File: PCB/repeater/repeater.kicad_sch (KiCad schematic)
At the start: 101 parts, among them J1 TX, J2 RX, J3 Conn_02x03_Counter_Clockwise, SW1 SW_Push, SW2 SW_SPDT, SW3 SW_SPDT, U1 DRA818V, U2 DRA818U, U3 PGA-103, U4 STM32F103C8Tx, U5 LMR33630ADDA, U6 AMS1117-3.3, U7 AMS1117-5.0, Y1 32.768KHz 12.5pF, Y2 8MHz 12pF

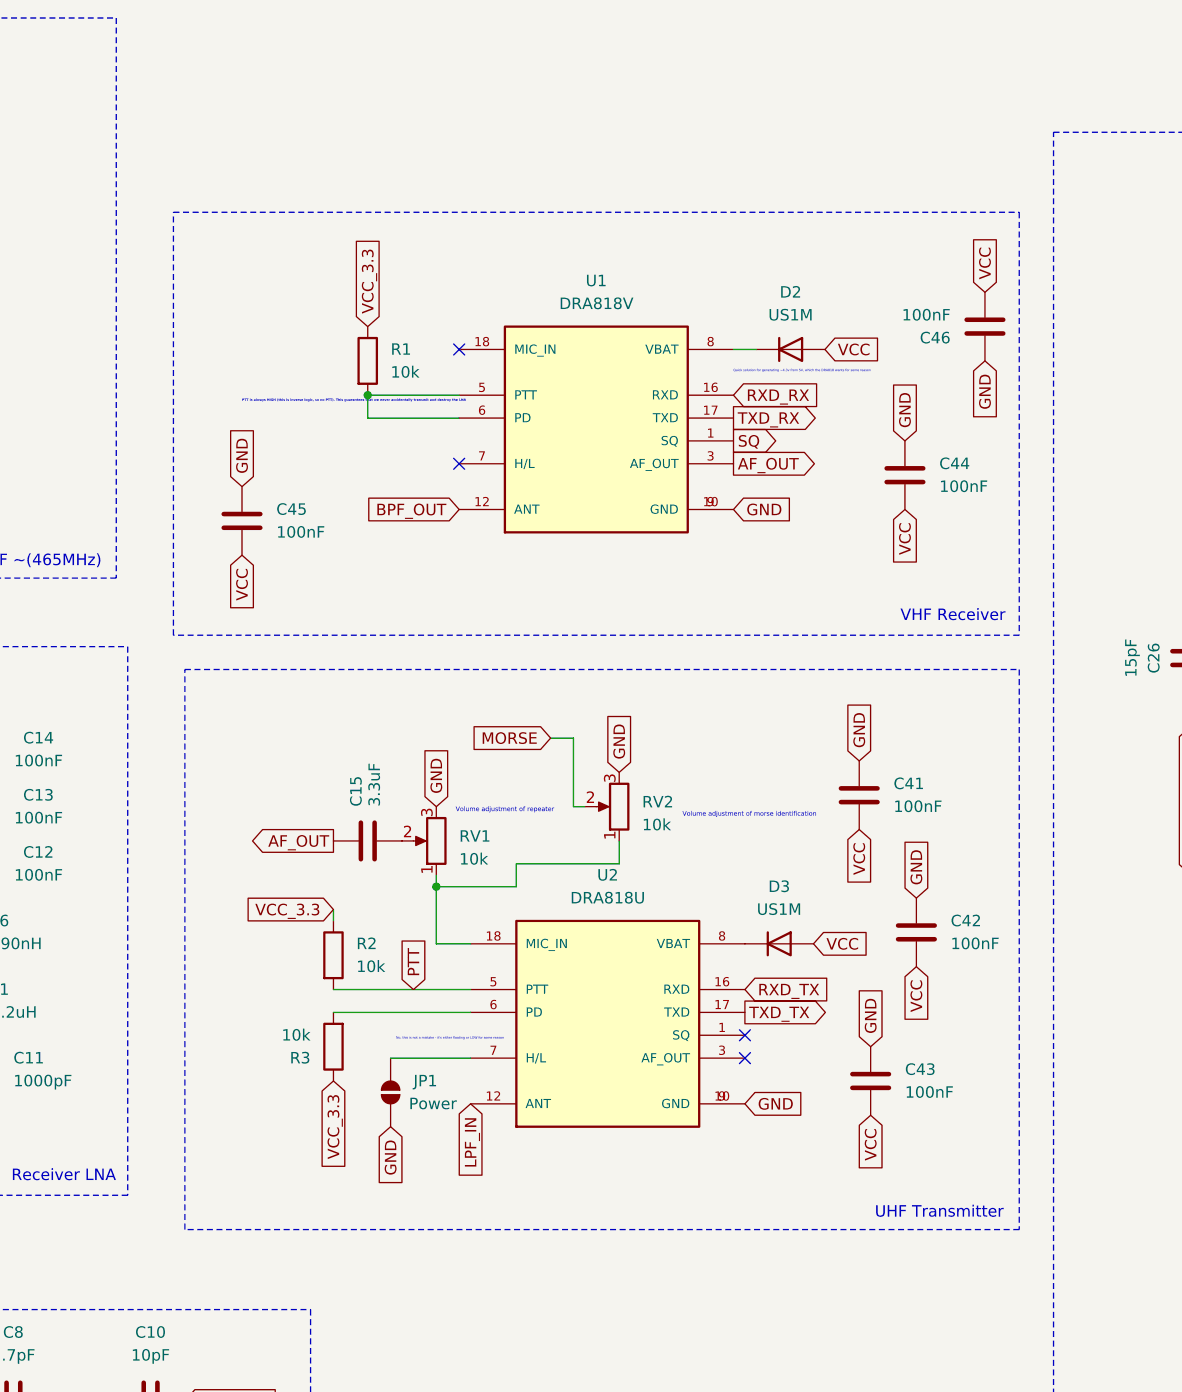
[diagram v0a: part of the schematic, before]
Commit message: Add filter and switch
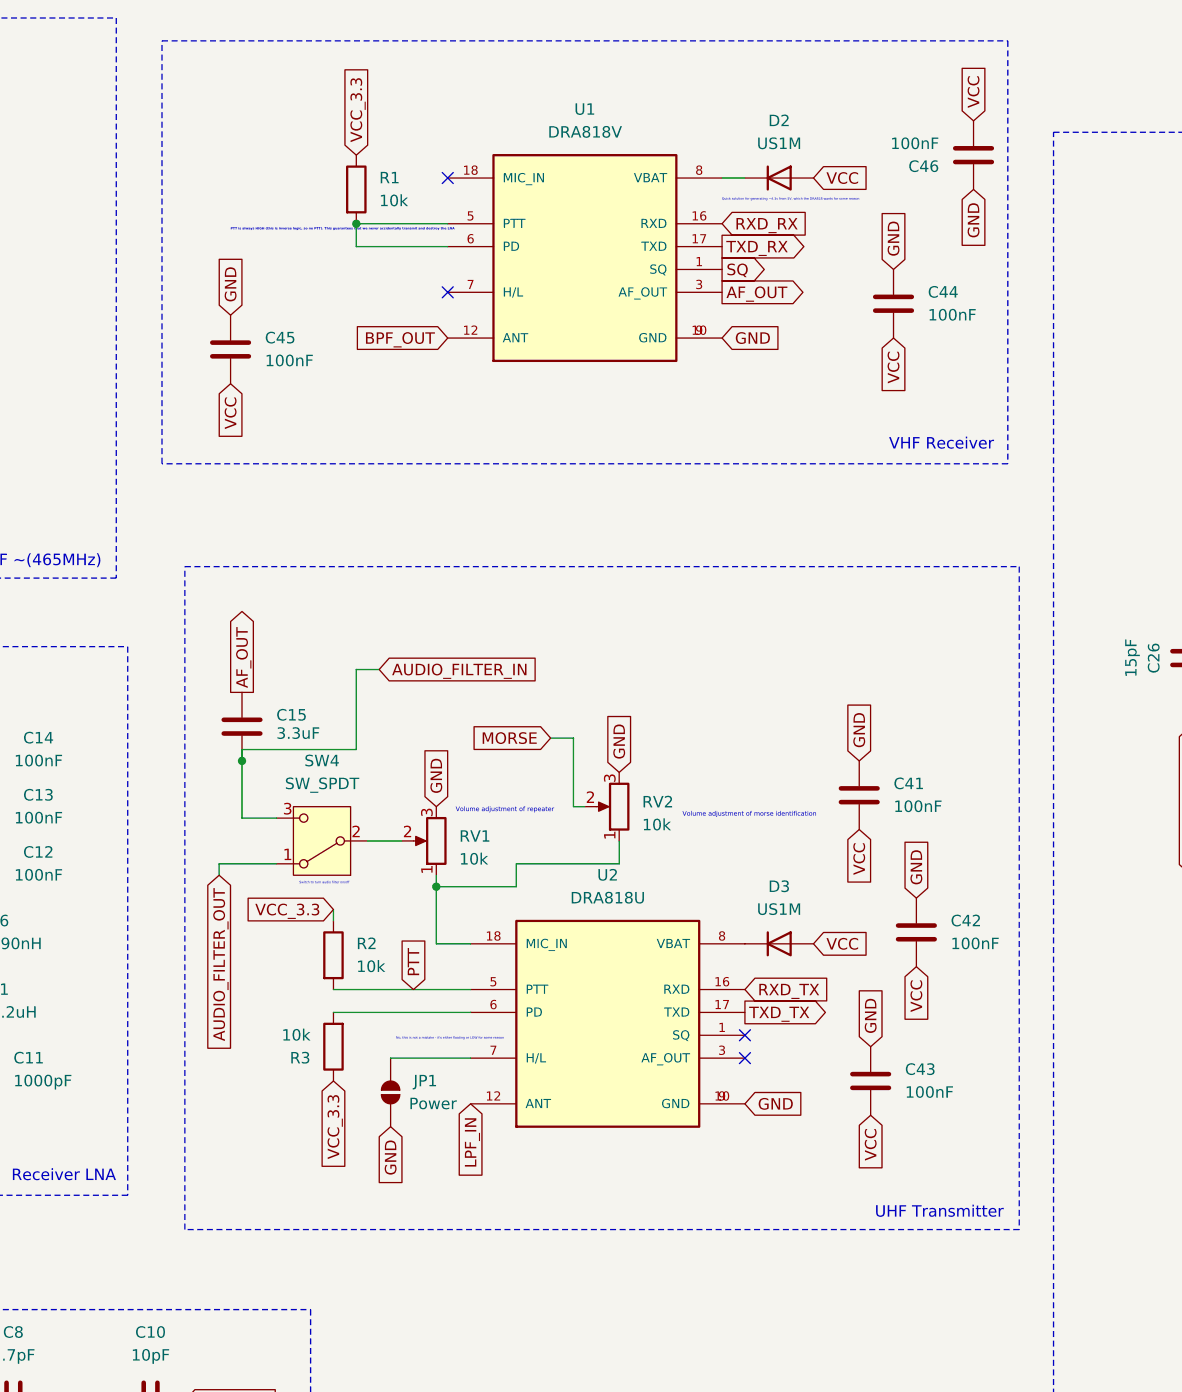
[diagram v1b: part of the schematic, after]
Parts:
- added SW4: SW_SPDT, symbol Switch:SW_SPDT
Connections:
- net AUDIO_FILTER_IN: now also C15.2, SW4.3 (C)
- net AUDIO_FILTER_OUT: now also SW4.1 (A)
- net at RV1.2: now also SW4.2 (B); no longer C15.2
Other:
- note added: "Switch to turn audio filter on/off"
- moved on the sheet: C15, C44, C45, C46, D2, R1, U1
